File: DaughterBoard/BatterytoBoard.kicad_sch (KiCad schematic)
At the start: 1 part, among them J1 705550019

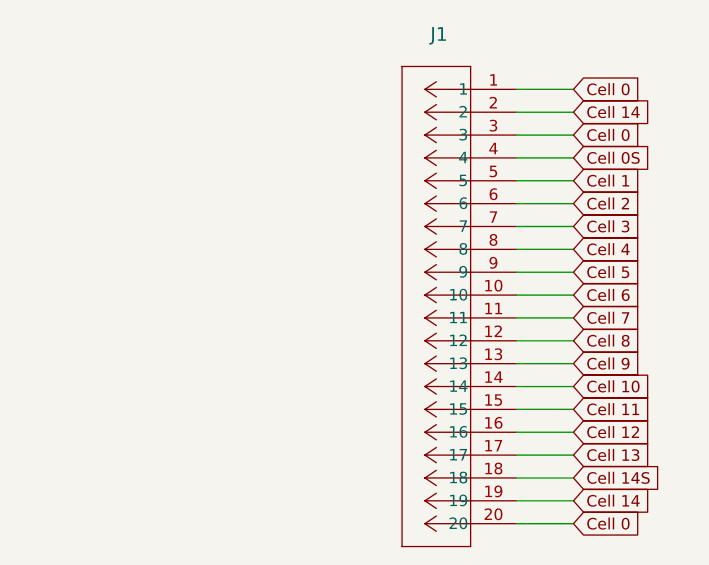
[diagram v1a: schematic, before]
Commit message: Connectors
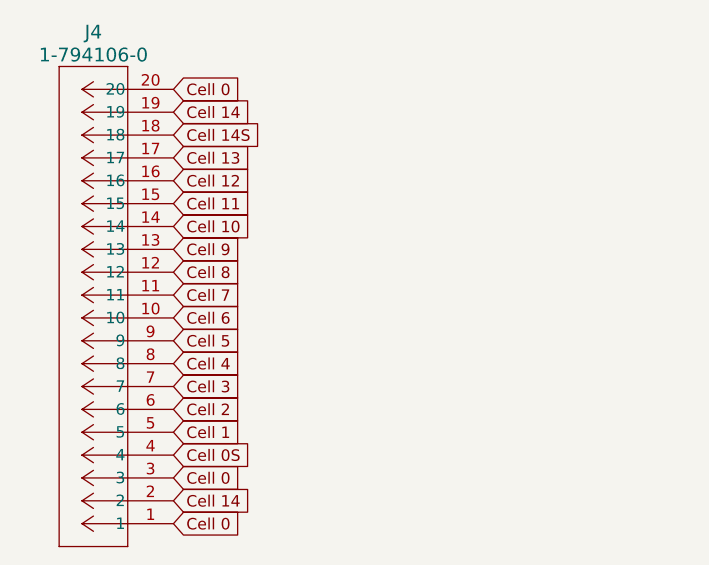
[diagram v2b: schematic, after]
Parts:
- removed J1: 705550019, 705550019:CONN_705550019_MOL, symbol 2024-10-07_23-48-39:705550019
- added J4: 1-794106-0, 1-794106-0:CON20_2X10_P4.14MM_RAMNL_TYC, symbol 1-794106-0:1-794106-0
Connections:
- net Cell 0: now also J4.1, J4.20, J4.3
- net Cell 0S: now also J4.4
- net Cell 1: now also J4.5
- net Cell 10: now also J4.14
- net Cell 11: now also J4.15
- net Cell 12: now also J4.16
- net Cell 13: now also J4.17
- net Cell 14: now also J4.19, J4.2
- net Cell 14S: now also J4.18
- net Cell 2: now also J4.6
- net Cell 3: now also J4.7
- net Cell 4: now also J4.8
- net Cell 5: now also J4.9
- net Cell 6: now also J4.10
- net Cell 7: now also J4.11
- net Cell 8: now also J4.12
- net Cell 9: now also J4.13
